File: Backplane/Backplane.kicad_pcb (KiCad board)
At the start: 2 copper layers, 100 x 90.3 mm, 6 parts, among them J1 0, J2 0

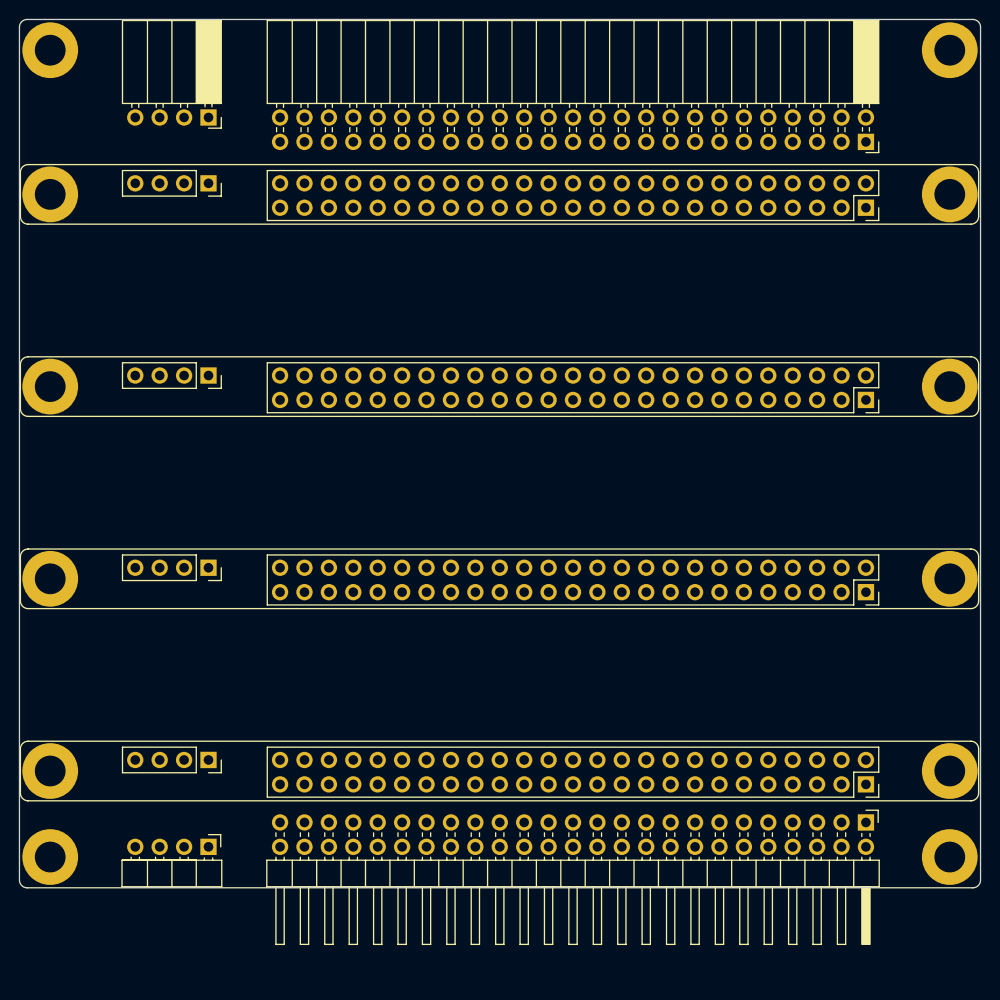
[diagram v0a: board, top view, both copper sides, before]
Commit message: a bunch of stuff
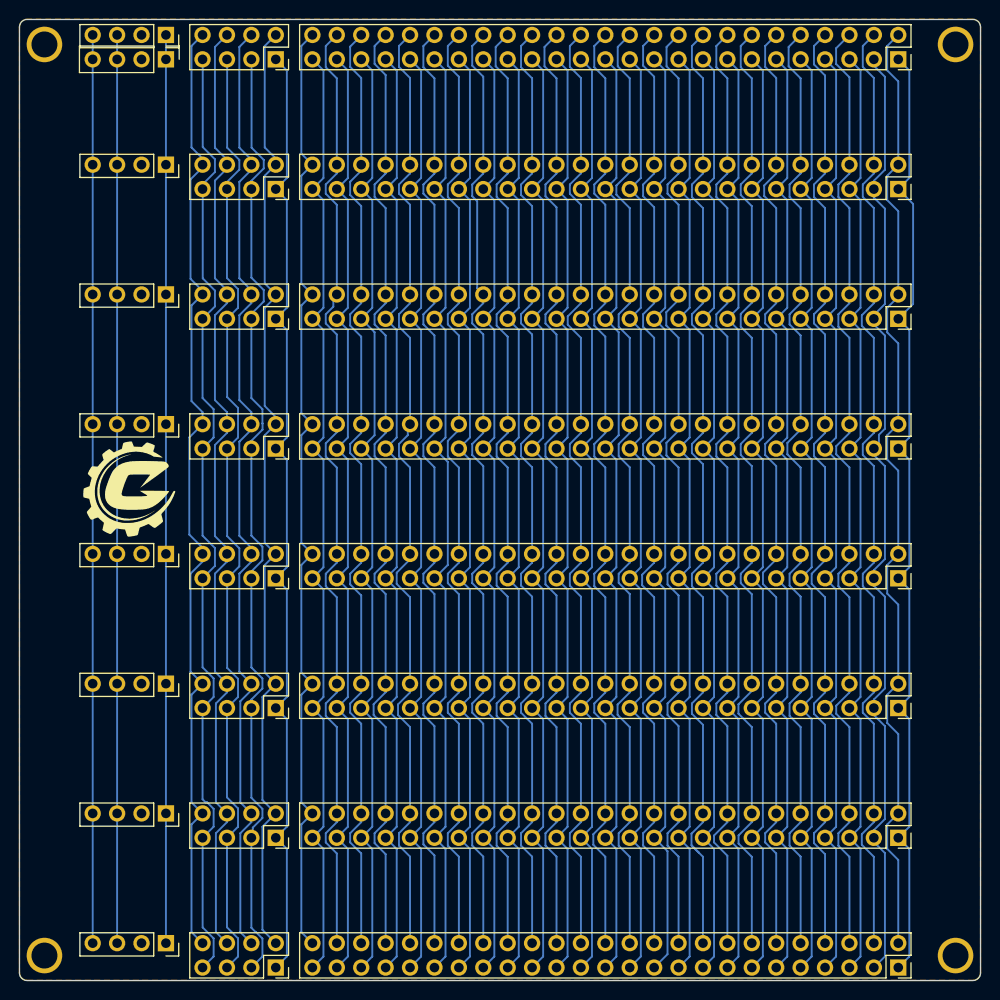
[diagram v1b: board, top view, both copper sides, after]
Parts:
- removed S0: 0, 0-Footprints:Slot
- removed S1: 1, 0-Footprints:Slot
- removed S2: 2, 0-Footprints:Slot
- removed S3: 3, 0-Footprints:Slot
- added G1: Logo, 0-Footprints:Crank, F.Cu at (36.5, 73.9)
- added H1: ~, 0-Footprints:MountingHolePadM2.5, F.Cu at (27.6, 27.6)
- added H2: ~, 0-Footprints:MountingHolePadM2.5, F.Cu at (122.4, 27.6)
- added H3: ~, 0-Footprints:MountingHolePadM2.5, F.Cu at (27.6, 122.4)
- added H4: ~, 0-Footprints:MountingHolePadM2.5, F.Cu at (122.4, 122.4)
- added J3: Slot 2, 0-Footprints:Slot, F.Cu at (25.0, 92.8)
- added J4: Slot 3, 0-Footprints:Slot, F.Cu at (25.0, 79.3)
- added J5: Slot 4, 0-Footprints:Slot, F.Cu at (25.0, 65.8)
- added J6: Slot 5, 0-Footprints:Slot, F.Cu at (25.0, 52.3)
- added J7: Slot 6, 0-Footprints:Slot, F.Cu at (25.0, 38.8)
- added J8: Slot 7, 0-Footprints:Slot, F.Cu at (25.0, 25.3)
- added J9: Power, 0-Footprints:PinHeader_1x04_P2.54mm_Vertical, F.Cu at (40.2, 29.1)
- J1: value 0 -> Slot 0; footprint 0-Footprints:BusInterconnect-F -> 0-Footprints:Slot
- J2: value 0 -> Slot 1; footprint 0-Footprints:BusInterconnect-M -> 0-Footprints:Slot
- moved J1 94.8 mm to (25.0, 119.8)
- moved J2 0.16 mm to (25.0, 106.3)
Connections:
- net /RAM_BANK0 renamed /P28
- net /RAM_BANK1 renamed /P30
- net /S1 renamed /~{RAM_SEL}
- net /S10 renamed /P20
- net /S11 renamed /P22
- net /S12 renamed /P24
- net /S13 renamed /P26
- net /S2 renamed /~{ROM_SEL}
- net /S3 renamed /~{BANK_SEL}
- net /S4 renamed /~{IO_SEL}
- net /S5 renamed /P10
- net /S6 renamed /P12
- net /S7 renamed /P14
- net /S8 renamed /P16
- net /S9 renamed /P18
- J1 pad 32: /~{TSC} -> /P32
- J1 pad 33: /R/~{W} -> /BUS_OK
- J1 pad 34: /DBE -> /P34
- J1 pad 36: /~{HALT} -> /P36
- J1 pad 38: /~{IRQ} -> /P38
- J1 pad 40: /~{NMI} -> /P40
- J1 pad 42: /~{RESET} -> /P42
- J1 pad 44: /Φ1 -> /P44
- J1 pad 46: /Φ2 -> /R/~{W}
- J1 pad 48: /BA -> /~{IRQ}
- J1 pad 50: /VMA -> /~{RESET}
- J2 pad 32: /~{TSC} -> /P32
- J2 pad 33: /R/~{W} -> /BUS_OK
- J2 pad 34: /DBE -> /P34
- J2 pad 36: /~{HALT} -> /P36
- J2 pad 38: /~{IRQ} -> /P38
- J2 pad 40: /~{NMI} -> /P40
- J2 pad 42: /~{RESET} -> /P42
- J2 pad 44: /Φ1 -> /P44
- J2 pad 46: /Φ2 -> /R/~{W}
- J2 pad 48: /BA -> /~{IRQ}
- J2 pad 50: /VMA -> /~{RESET}
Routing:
- net /P18: track 0.00 -> 102.2 mm
- net /~{BANK_SEL}: track 0.00 -> 101.7 mm
- net /P14: track 0.00 -> 101.6 mm
- net /P24: track 0.00 -> 101.6 mm
- net /A0: track 0.00 -> 101.5 mm
- net /A12: track 0.00 -> 101.4 mm
- net /D5: track 0.00 -> 101.4 mm
- net /P16: track 0.00 -> 101.4 mm
- net /D2: track 0.00 -> 101.4 mm
- net /A10: track 0.00 -> 101.4 mm
- net /P28: track 0.00 -> 101.4 mm
- net /~{ROM_SEL}: track 0.00 -> 101.3 mm
- net /P22: track 0.00 -> 101.3 mm
- net /P44: track 0.00 -> 101.3 mm
- net /P26: track 0.00 -> 101.3 mm
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- added copper zone on F.Cu, net GND
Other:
- board size 100 x 90.3 mm -> 100 x 100 mm
